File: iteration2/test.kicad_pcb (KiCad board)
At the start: 2 copper layers, 133.3 x 128.6 mm, 95 parts, among them U1 Raspberry_Pi_Pico

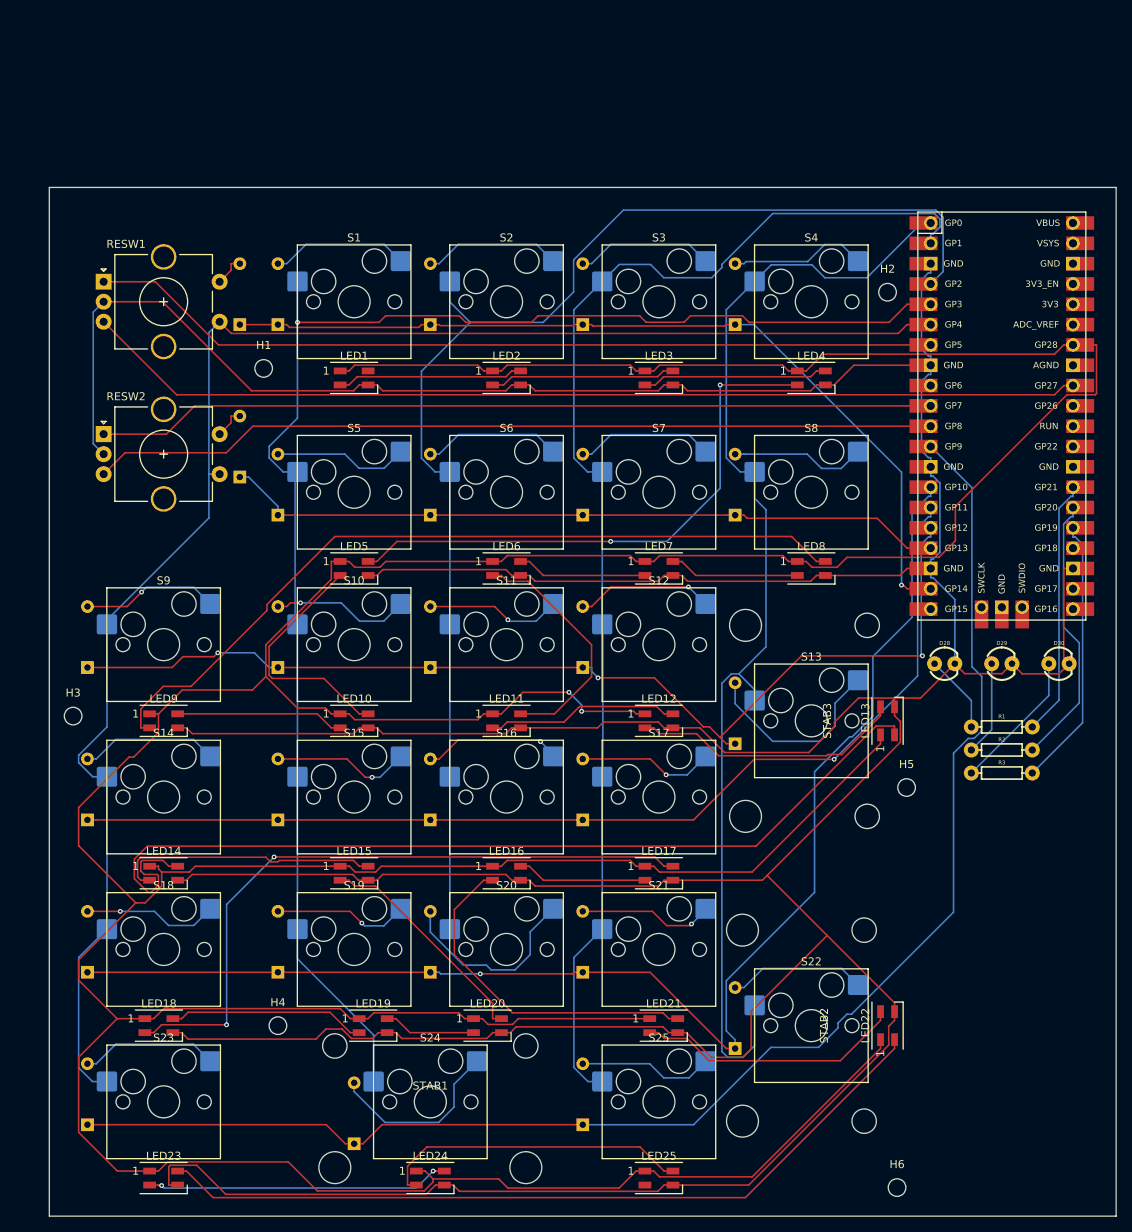
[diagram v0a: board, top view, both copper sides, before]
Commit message: update layout
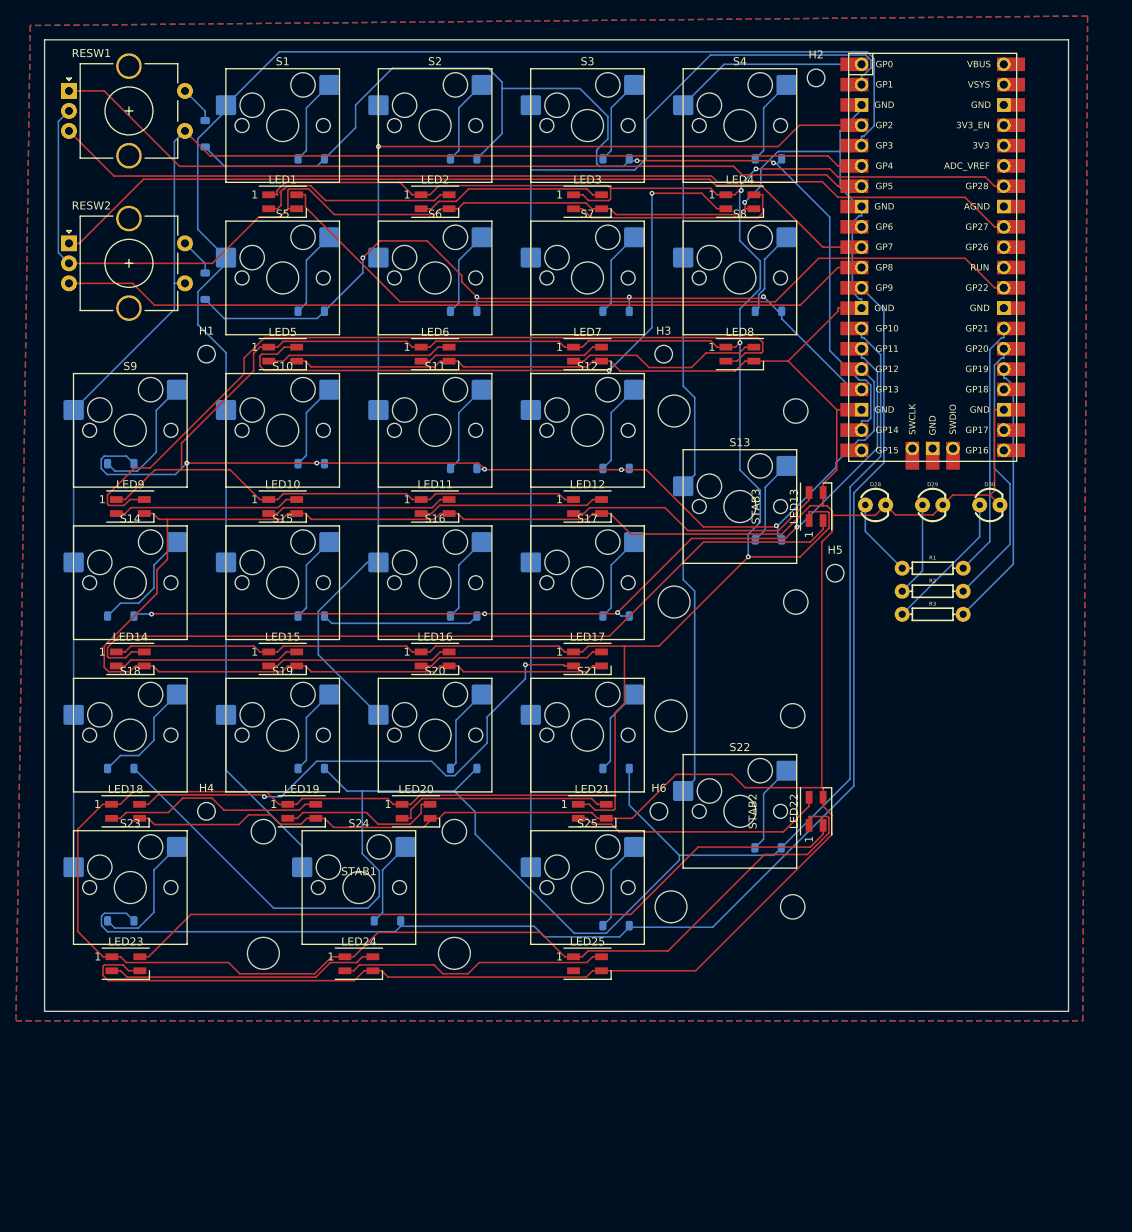
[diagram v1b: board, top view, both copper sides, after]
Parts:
- D1, D10, D11, D12, D13, D14, D15, D16, D17, D18, D19, D2, D20, D21, D22, D23, D24, D25, D26, D27, D3, D4, D5, D6, D7, D8, D9: footprint ScottoKeebs_Components:Diode_DO-35 -> Diode_SMD:D_SOD-123
- moved H3 86.6 mm to (100.6, 58.9)
- moved H6 55.7 mm to (100.0, 116.1)
- moved H4 28.2 mm to (43.5, 116.1)
- moved LED10 28.2 mm to (53.0, 78.0)
- moved LED11 28.2 mm to (72.0, 78.0)
- moved LED13 28.2 mm to (119.7, 78.0)
- moved LED15 28.2 mm to (53.0, 97.0)
- moved LED16 28.2 mm to (72.0, 97.0)
- moved LED19 28.2 mm to (55.4, 116.1)
- moved LED22 28.2 mm to (119.7, 116.1)
- moved S10 28.2 mm to (53.0, 68.5)
- moved S11 28.2 mm to (72.0, 68.5)
- moved S5 28.2 mm to (53.0, 49.4)
- moved S6 28.2 mm to (72.0, 49.4)
- moved H2 28.2 mm to (119.7, 24.4)
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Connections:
- LED11 pad 4: Net-(LED11-DIN) -> Net-(LED10-DOUT)
- LED16 pad 4: Net-(LED16-DIN) -> Net-(LED15-DOUT)
- LED17 pad 2: Net-(LED16-DIN) -> Net-(LED17-DOUT)
- LED17 pad 4: Net-(LED17-DIN) -> Net-(LED16-DOUT)
- LED18 pad 2: Net-(LED17-DIN) -> Net-(LED18-DOUT)
- LED18 pad 4: Net-(LED18-DIN) -> Net-(LED17-DOUT)
- LED19 pad 2: Net-(LED18-DIN) -> Net-(LED19-DOUT)
- LED19 pad 4: Net-(LED19-DIN) -> Net-(LED18-DOUT)
- LED20 pad 2: Net-(LED19-DIN) -> Net-(LED20-DOUT)
- LED20 pad 4: Net-(LED15-DOUT) -> Net-(LED19-DOUT)
- LED21 pad 4: Net-(LED16-DOUT) -> Net-(LED20-DOUT)
- LED5 pad 2: Net-(LED10-DIN) -> Net-(LED5-DOUT)
- LED6 pad 2: Net-(LED11-DIN) -> Net-(LED6-DOUT)
- LED6 pad 4: Net-(LED6-DIN) -> Net-(LED5-DOUT)
- LED7 pad 2: Net-(LED6-DIN) -> Net-(LED7-DOUT)
- LED7 pad 4: Net-(LED7-DIN) -> Net-(LED6-DOUT)
- LED8 pad 2: Net-(LED7-DIN) -> Net-(LED8-DOUT)
- LED8 pad 4: Net-(LED8-DIN) -> Net-(LED7-DOUT)
- LED9 pad 2: Net-(LED8-DIN) -> Net-(LED10-DIN)
- LED9 pad 4: Net-(LED10-DOUT) -> Net-(LED8-DOUT)
- U1 pad 29: unconnected-(U1-GPIO22-Pad29) -> /KEY_LEDS
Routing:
- net Net-(LED8-DOUT): track 0.00 -> 103.8 mm
- net Net-(LED8-DIN): track 99.7 -> 0.00 mm
- net /KEY_LEDS: track 0.00 -> 98.6 mm
- net Net-(LED17-DIN): track 84.4 -> 0.00 mm, vias 2 -> 0
- net Net-(LED17-DOUT): track 0.00 -> 66.2 mm, vias 0 -> 2
- net Row1: track 166.6 -> 213.3 mm, vias 1 -> 0
- net VCC: track 659.6 -> 619.9 mm, vias 2 -> 4
- net Row5: track 108.8 -> 141.4 mm, vias 1 -> 2
- net Col4: track 144.2 -> 112.5 mm
- net Net-(LED11-DIN): track 30.8 -> 0.00 mm
- net Net-(LED18-DOUT): track 0.00 -> 27.5 mm
- net Net-(LED20-DOUT): track 0.00 -> 27.5 mm
- net Net-(LED18-DIN): track 24.7 -> 0.00 mm
- net Net-(LED7-DOUT): track 0.00 -> 24.5 mm
- net Net-(LED6-DOUT): track 0.00 -> 23.3 mm
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- added copper zone on B.Cu, net (none)
- added copper zone on F.Cu, net (none)
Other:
- board size 133.3 x 128.6 mm -> 128 x 121.4 mm
